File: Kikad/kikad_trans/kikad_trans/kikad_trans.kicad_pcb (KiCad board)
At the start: 2 copper layers, 13 parts

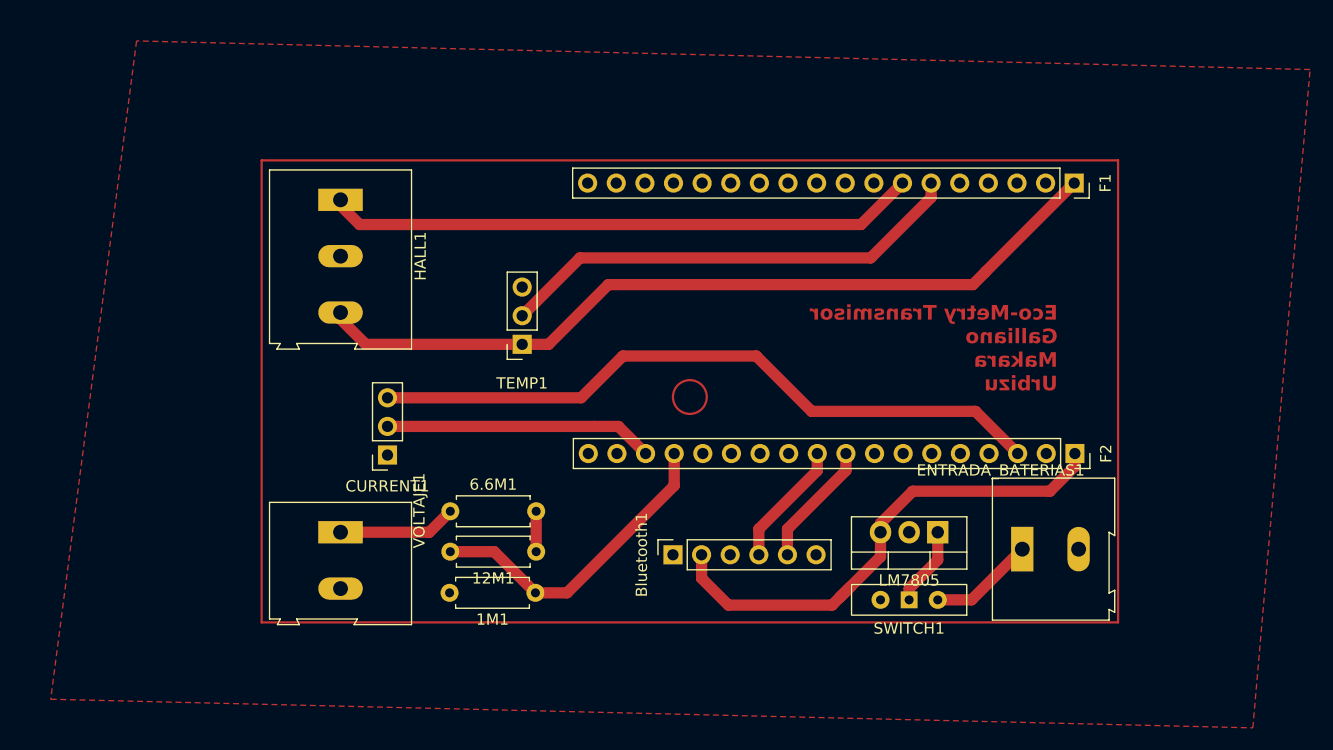
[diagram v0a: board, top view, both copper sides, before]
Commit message: Kikad ahora si
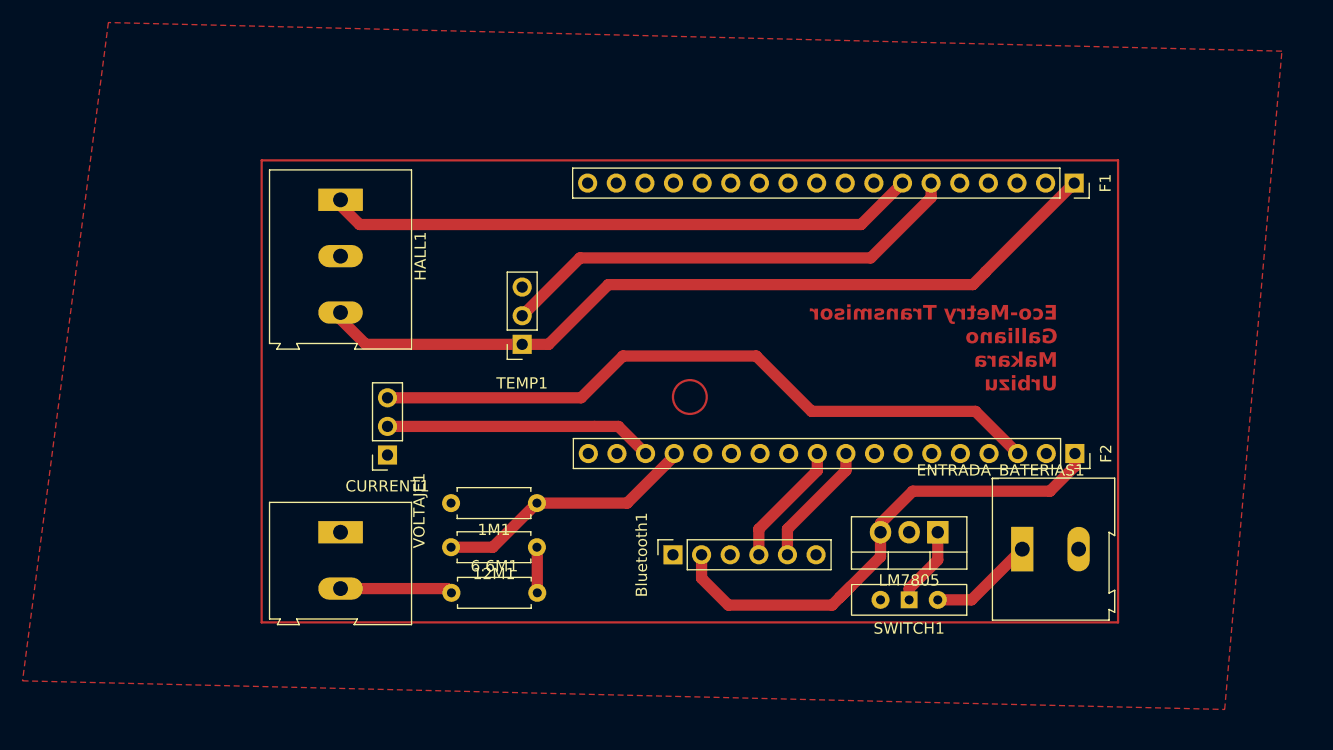
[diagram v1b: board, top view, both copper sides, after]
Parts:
- moved 1M1 7.96 mm to (124.4, 129.9)
- moved 6.6M1 7.24 mm to (116.8, 137.9)
- moved 12M1 0.40 mm to (124.4, 133.8)
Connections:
- 6.6M1 pad 1: Net-(VOLTAJE1-Pin_1) -> Net-(VOLTAJE1-Pin_2)
- VOLTAJE1 pad 1: Net-(VOLTAJE1-Pin_1) -> GND
- VOLTAJE1 pad 2: GND -> Net-(VOLTAJE1-Pin_2)
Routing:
- net Net-(VOLTAJE1-Pin_1): track 10.5 -> 0.00 mm
- net Net-(VOLTAJE1-Pin_2): track 0.00 -> 10.00 mm
- net Net-(F2-Pin_15): track 28.2 -> 23.4 mm
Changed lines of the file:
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@@
 	(net 5 "Net-(Bluetooth1-Pin_4)")
 	(net 6 "Net-(Bluetooth1-Pin_5)")
-	(net 7 "Net-(VOLTAJE1-Pin_1)")
+	(net 7 "Net-(VOLTAJE1-Pin_2)")
 	(net 8 "Net-(CURRENT1-Pin_2)")
 	(net 9 "3.3V")
@@
 	(footprint "Resistor_THT:R_Axial_DIN0207_L6.3mm_D2.5mm_P7.62mm_Horizontal"
 		(layer "F.Cu")
-		(at 116.742495 130.638147)
+		(at 116.841219 137.877879)
 		(descr "Resistor, Axial_DIN0207 series, Axial, Horizontal, pin pitch=7.62mm, 0.25W = 1/4W, length*diameter=6.3*2.5mm^2, http://cdn-reichelt.de/documents/datenblatt/B400/1_4W%23YAG.pdf")
 		(tags "Resistor Axial_DIN0207 series Axial Horizontal pin pitch 7.62mm 0.25W = 1/4W length 6.3mm diameter 2.5mm")
@@
 			(layers "*.Cu" "*.Mask")
 			(remove_unused_layers no)
-			(net 7 "Net-(VOLTAJE1-Pin_1)")
+			(net 7 "Net-(VOLTAJE1-Pin_2)")
 			(pintype "passive")
 		)
@@
 			(layers "*.Cu" "*.Mask")
 			(remove_unused_layers no)
-			(net 7 "Net-(VOLTAJE1-Pin_1)")
+			(net 4 "GND")
 			(pinfunction "Pin_1")
 			(pintype "passive")
@@
 			(layers "*.Cu" "*.Mask")
 			(remove_unused_layers no)
-			(net 4 "GND")
+			(net 7 "Net-(VOLTAJE1-Pin_2)")
 			(pinfunction "Pin_2")
 			(pintype "passive")
@@
 	(footprint "Resistor_THT:R_Axial_DIN0207_L6.3mm_D2.5mm_P7.62mm_Horizontal"
 		(layer "F.Cu")
-		(at 124.362495 134.225105 180)
+		(at 124.428311 133.830211 180)
 		(descr "Resistor, Axial_DIN0207 series, Axial, Horizontal, pin pitch=7.62mm, 0.25W = 1/4W, length*diameter=6.3*2.5mm^2, http://cdn-reichelt.de/documents/datenblatt/B400/1_4W%23YAG.pdf")
 		(tags "Resistor Axial_DIN0207 series Axial Horizontal pin pitch 7.62mm 0.25W = 1/4W length 6.3mm diameter 2.5mm")
@@
 	(footprint "Resistor_THT:R_Axial_DIN0207_L6.3mm_D2.5mm_P7.62mm_Horizontal"
 		(layer "F.Cu")
-		(at 124.296679 137.877879 180)
+		(at 124.428311 129.914174 180)
 		(descr "Resistor, Axial_DIN0207 series, Axial, Horizontal, pin pitch=7.62mm, 0.25W = 1/4W, length*diameter=6.3*2.5mm^2, http://cdn-reichelt.de/documents/datenblatt/B400/1_4W%23YAG.pdf")
 		(tags "Resistor Axial_DIN0207 series Axial Horizontal pin pitch 7.62mm 0.25W = 1/4W length 6.3mm diameter 2.5mm")
@@
 	)
 	(segment
-		(start 114.880642 132.5)
-		(end 116.742495 130.638147)
+		(start 107 137.5)
+		(end 116.46334 137.5)
 		(width 1)
 		(layer "F.Cu")
@@
 	)
 	(segment
-		(start 107 132.5)
-		(end 114.880642 132.5)
+		(start 116.46334 137.5)
+		(end 116.841219 137.877879)
 		(width 1)
 		(layer "F.Cu")
@@
 	)
 	(segment
-		(start 124.362495 130.638147)
-		(end 124.362495 134.225105)
+		(start 124.461219 133.863119)
+		(end 124.428311 133.830211)
+		(width 1)
+		(layer "F.Cu")
+		(net 17)
+	)
+	(segment
+		(start 124.461219 137.877879)
+		(end 124.461219 133.863119)
 		(width 1)
 		(layer "F.Cu")
@@
 	)
 	(segment
-		(start 120.643905 134.225105)
-		(end 124.296679 137.877879)
+		(start 136.609704 125.740973)
+		(end 136.609704 125.515795)
 		(width 1)
 		(layer "F.Cu")
@@
 	)
 	(segment
-		(start 136.609704 128.369336)
-		(end 127.101161 137.877879)
+		(start 124.428311 129.914174)
+		(end 132.436503 129.914174)
 		(width 1)
 		(layer "F.Cu")
@@
 	)
 	(segment
-		(start 116.742495 134.225105)
-		(end 120.643905 134.225105)
+		(start 116.808311 133.830211)
+		(end 120.512274 133.830211)
 		(width 1)
 		(layer "F.Cu")
@@
 	)
 	(segment
-		(start 136.609704 125.515795)
-		(end 136.609704 128.369336)
+		(start 132.436503 129.914174)
+		(end 136.609704 125.740973)
 		(width 1)
 		(layer "F.Cu")
@@
 	)
 	(segment
-		(start 124.296679 137.877879)
-		(end 127.101161 137.877879)
+		(start 120.512274 133.830211)
+		(end 124.428311 129.914174)
 		(width 1)
 		(layer "F.Cu")
@@
 		(polygon
 			(pts
-				(xy 88.9 88.9) (xy 81.28 147.32) (xy 187.96 149.86) (xy 193.04 91.44)
+				(xy 86.400149 87.268099) (xy 78.780149 145.688099) (xy 185.460149 148.228099) (xy 190.540149 89.808099)
 			)
 		)

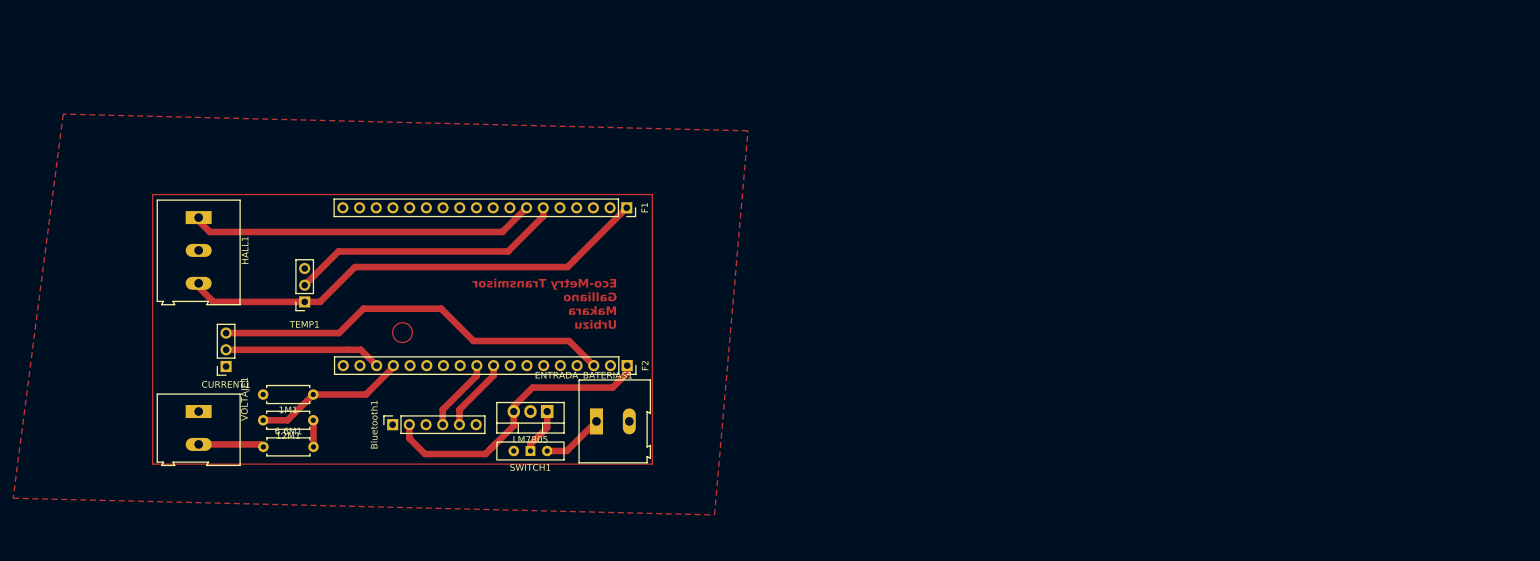
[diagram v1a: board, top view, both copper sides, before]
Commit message: ahora si lcdtm
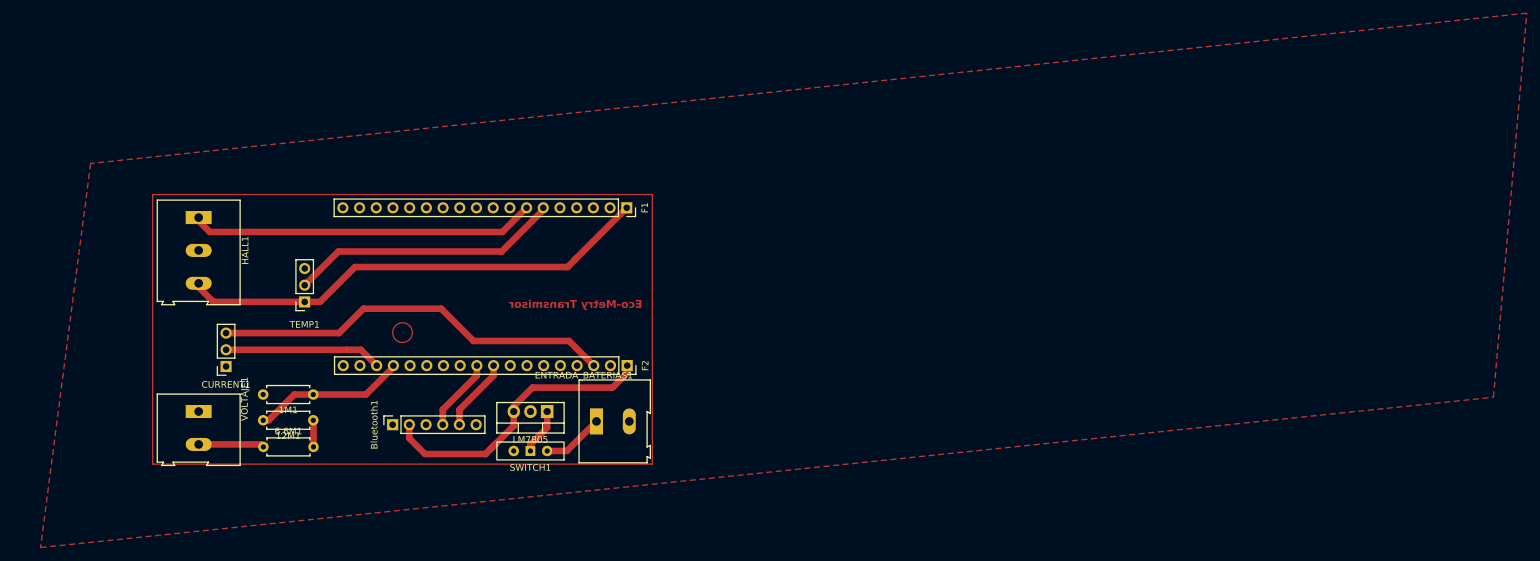
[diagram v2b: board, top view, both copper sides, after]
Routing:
- net Net-(F1-Pin_6): track 41.9 -> 41.4 mm
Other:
- board text added: "Eco-Metry Transmisor"
- board text removed: "Eco-Metry Transmisor Galliano Makara Urbizu"
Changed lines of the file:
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@@
 		(layer "F.Cu")
 	)
-	(gr_text "Eco-Metry Transmisor\nGalliano\nMakara\nUrbizu"
-		(at 170.643454 120.068932 0)
-		(layer "F.Cu" knockout)
+	(gr_text "Eco-Metry Transmisor"
+		(at 174.478743 116.885095 0)
+		(layer "F.Cu")
 		(effects
 			(font
-				(size 1.3 1.3)
+				(size 1.2 1.2)
 				(thickness 0.26)
 				(bold yes)
@@
 	)
 	(segment
-		(start 159.409704 102.798371)
-		(end 154.051487 108.156588)
+		(start 128.250192 108.156588)
+		(end 123.120831 113.285949)
 		(width 1)
 		(layer "F.Cu")
@@
 	)
 	(segment
-		(start 128.250192 108.156588)
-		(end 154.051487 108.156588)
+		(start 159.409704 101.839776)
+		(end 153.092892 108.156588)
 		(width 1)
 		(layer "F.Cu")
@@
 	)
 	(segment
-		(start 123.120831 113.285949)
+		(start 153.092892 108.156588)
 		(end 128.250192 108.156588)
 		(width 1)
@@
 	(segment
 		(start 159.409704 101.515795)
-		(end 159.409704 102.798371)
+		(end 159.409704 101.839776)
 		(width 1)
 		(layer "F.Cu")
@@
 	)
 	(segment
+		(start 116.808311 133.830211)
+		(end 117.629789 133.830211)
+		(width 1)
+		(layer "F.Cu")
+		(net 18)
+	)
+	(segment
 		(start 136.609704 125.740973)
 		(end 136.609704 125.515795)
@@
 	)
 	(segment
+		(start 121.545826 129.914174)
+		(end 124.428311 129.914174)
+		(width 1)
+		(layer "F.Cu")
+		(net 18)
+	)
+	(segment
 		(start 124.428311 129.914174)
 		(end 132.436503 129.914174)
@@
 	)
 	(segment
-		(start 116.808311 133.830211)
-		(end 120.512274 133.830211)
-		(width 1)
-		(layer "F.Cu")
-		(net 18)
-	)
-	(segment
 		(start 132.436503 129.914174)
 		(end 136.609704 125.740973)
@@
 	)
 	(segment
-		(start 120.512274 133.830211)
-		(end 124.428311 129.914174)
+		(start 117.629789 133.830211)
+		(end 121.545826 129.914174)
 		(width 1)
 		(layer "F.Cu")
@@
 		(polygon
 			(pts
-				(xy 86.400149 87.268099) (xy 78.780149 145.688099) (xy 185.460149 148.228099) (xy 190.540149 89.808099)
+				(xy 90.564094 94.768614) (xy 82.944094 153.188614) (xy 303.924094 130.328614) (xy 309.004094 71.908614)
 			)
 		)
